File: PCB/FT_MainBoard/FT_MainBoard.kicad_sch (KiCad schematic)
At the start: 7 parts

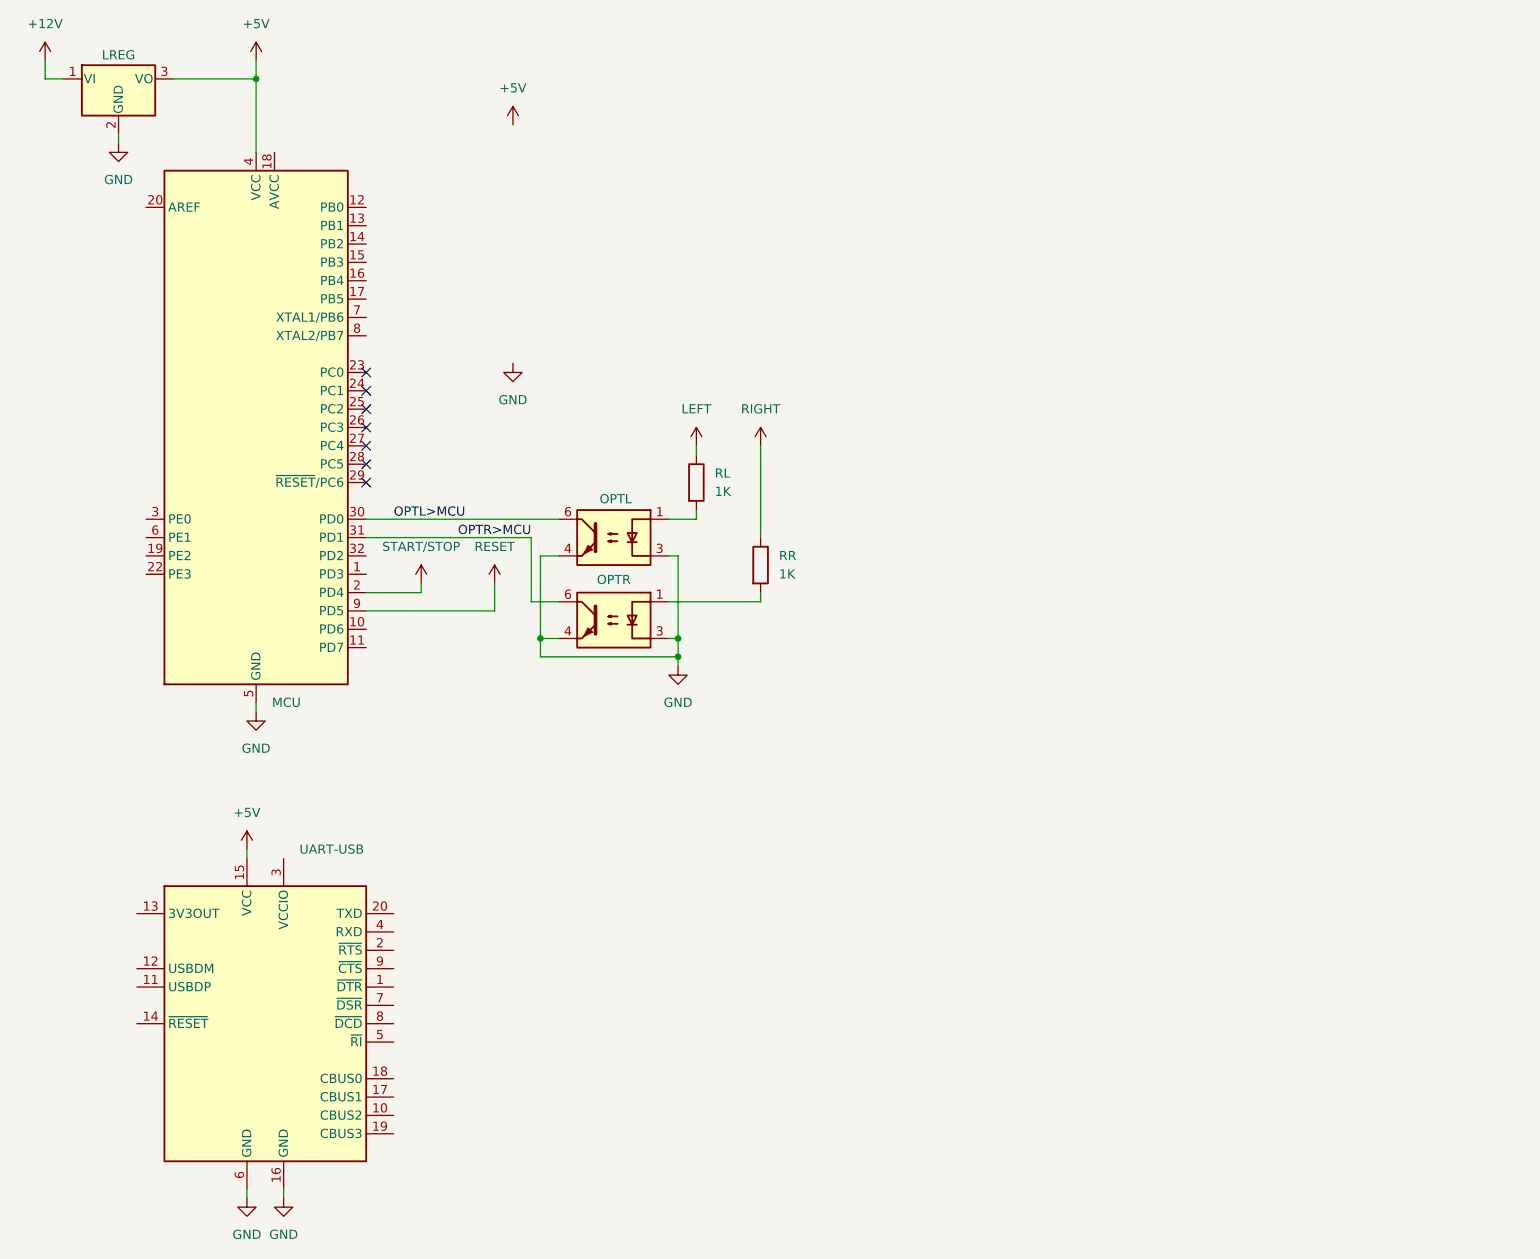
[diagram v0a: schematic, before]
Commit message: update mb shematic
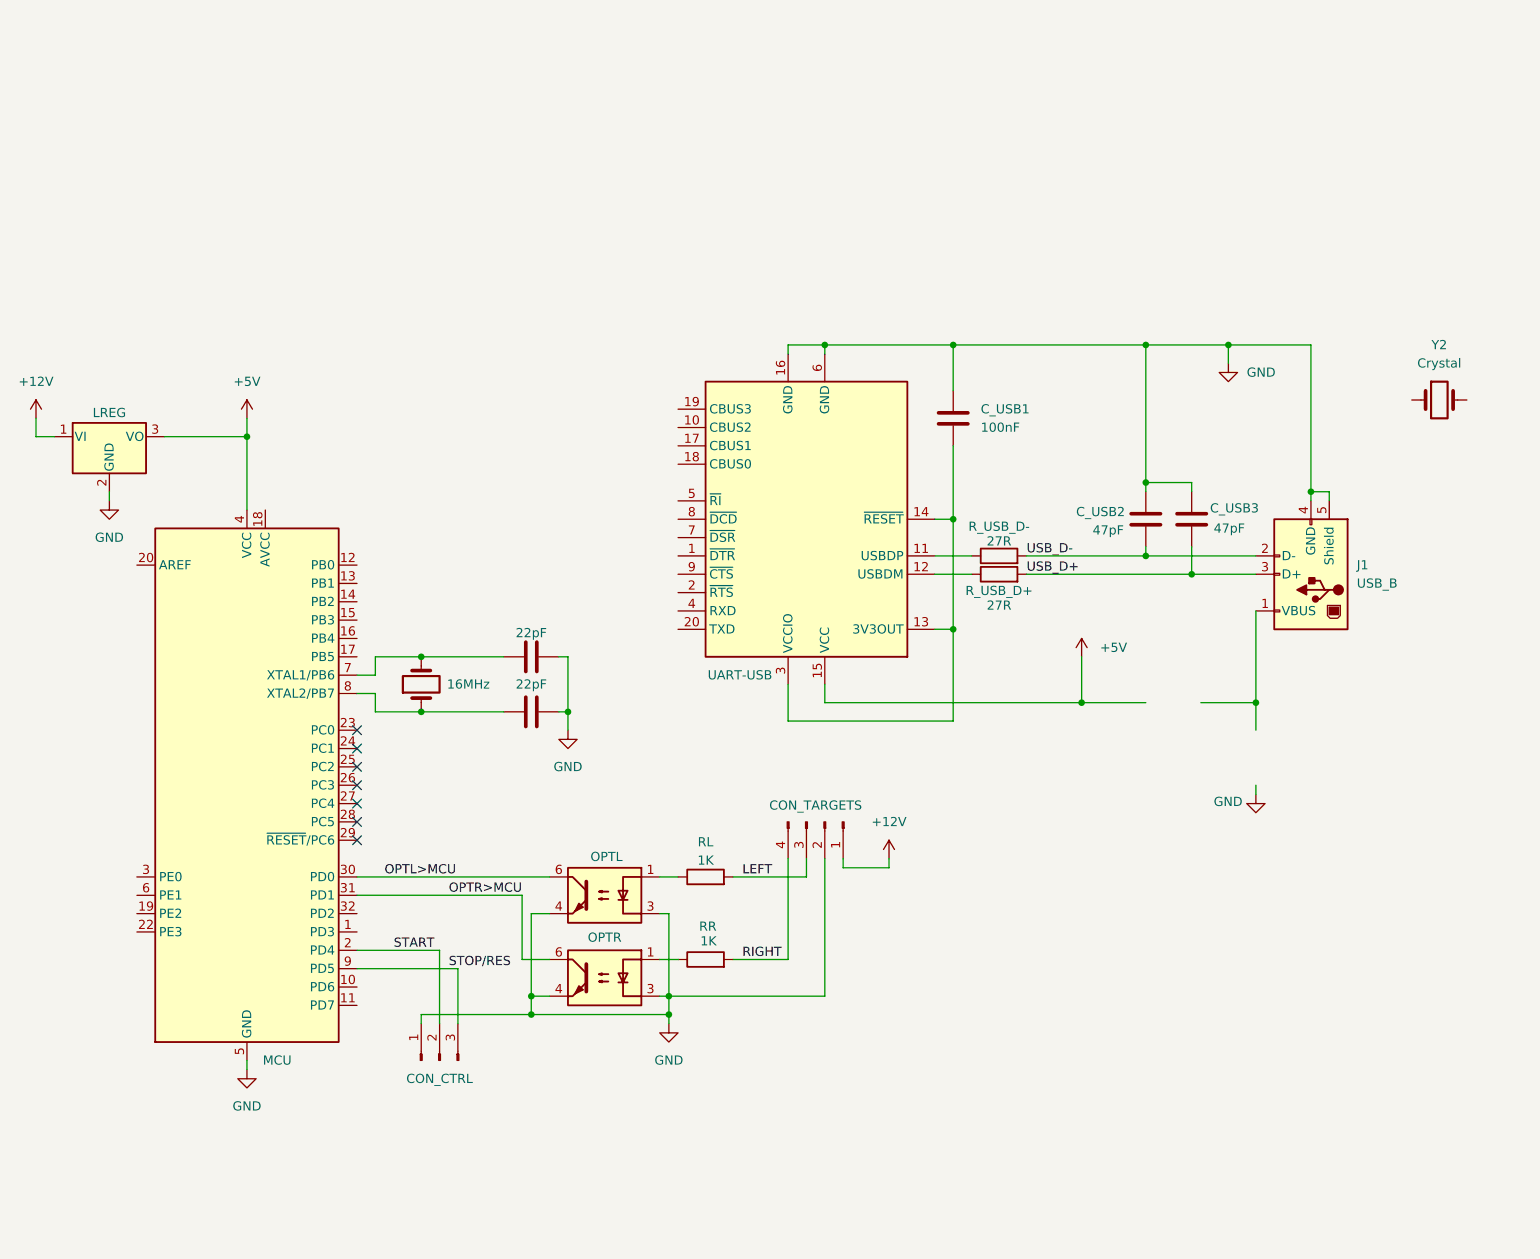
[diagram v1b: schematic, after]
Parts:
- added CON_CTRL: Conn_01x03_Pin, Connector:FanPinHeader_1x03_P2.54mm_Vertical, symbol Connector:Conn_01x03_Pin
- added CON_TARGETS: Conn_01x04_Pin, Connector:FanPinHeader_1x04_P2.54mm_Vertical, symbol Connector:Conn_01x04_Pin
- added C_MCU_OSC1, C_MCU_OSC2: 22pF, symbol Device:C
- added C_USB1: 100nF, symbol Device:C
- added C_USB2, C_USB3: 47pF, symbol Device:C
- added J1: USB_B, symbol Connector:USB_B
- added MCU_OSC: 16MHz, Crystal:Crystal_SMD_HC49-SD_HandSoldering, symbol Device:Crystal
- added R_USB_D+, R_USB_D-: 27R, symbol Device:R
- added Y2: Crystal, Crystal:Crystal_SMD_HC49-SD_HandSoldering, symbol Device:Crystal
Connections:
- net +12V: now also CON_TARGETS.1 (Pin_1)
- net GND: now also CON_CTRL.1 (Pin_1), CON_TARGETS.2 (Pin_2), C_MCU_OSC1.2, C_MCU_OSC2.2, C_USB1.1, C_USB2.1, C_USB3.1, J1.4 (GND), J1.5 (Shield)
- net LEFT: now also RL.2, CON_TARGETS.3 (Pin_3); no longer RL.1
- net RIGHT: now also RR.2, CON_TARGETS.4 (Pin_4); no longer RR.1
- net at OPTL.1: now also RL.1; no longer RL.2
- net at OPTR.1: now also RR.1; no longer RR.2
- net at MCU.7 (XTAL1/PB6): now also C_MCU_OSC1.1, MCU_OSC.2
- net at MCU.8 (XTAL2/PB7): now also C_MCU_OSC2.1, MCU_OSC.1
- net at UART-USB.11 (USBDP): now also R_USB_D-.1
- net at UART-USB.12 (USBDM): now also R_USB_D+.1
- net at UART-USB.13 (3V3OUT): now also UART-USB.14 (~{RESET}), UART-USB.3 (VCCIO), C_USB1.2
- net RESET renamed STOP/RES
- net STOP/RES: now also CON_CTRL.3 (Pin_3)
- net START/STOP renamed START
- net START: now also CON_CTRL.2 (Pin_2)
- new net USB_D+: C_USB3.2, J1.3 (D+), R_USB_D+.2
- new net USB_D-: C_USB2.2, J1.2 (D-), R_USB_D-.2
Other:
- moved on the sheet: LREG, MCU, OPTL, OPTR, RL, RR, UART-USB

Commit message: main board corruption fix
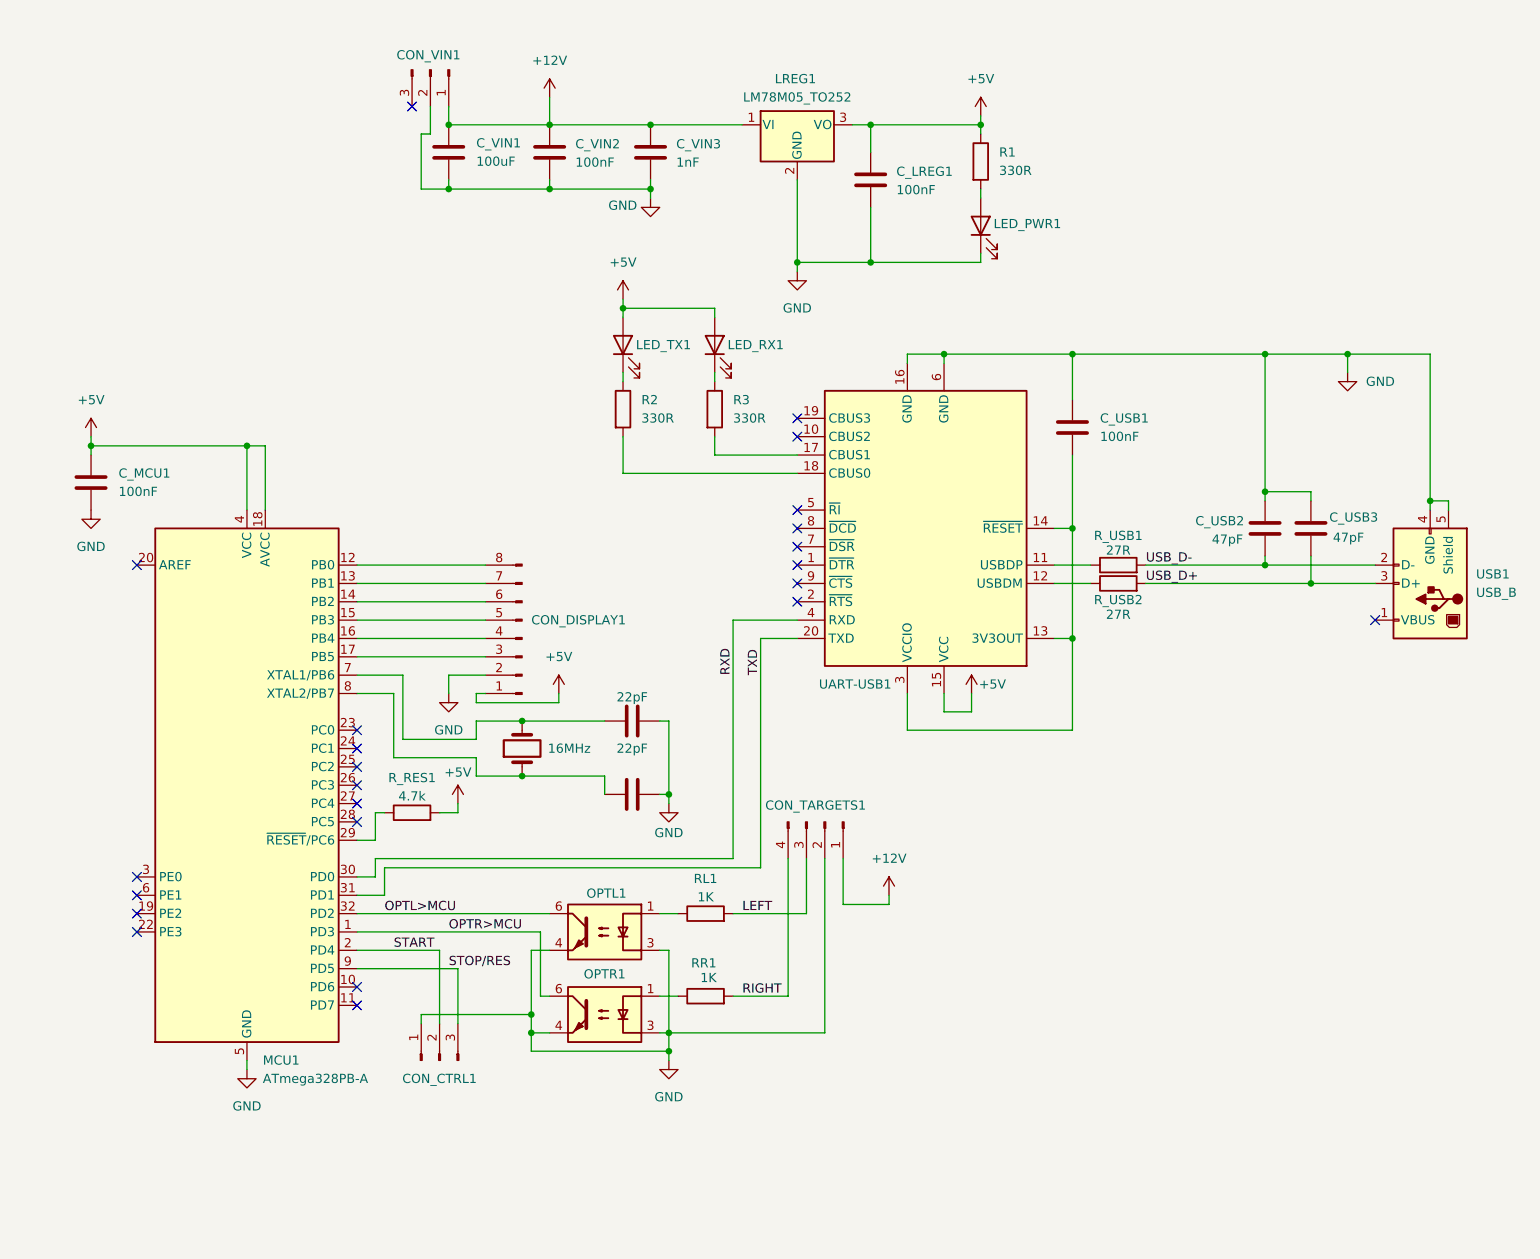
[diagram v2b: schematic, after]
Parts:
- removed Y2: Crystal, Crystal:Crystal_SMD_HC49-SD_HandSoldering, symbol Device:Crystal
- added CON_DISPLAY1: Conn_01x08_Pin, Connector_PinSocket_2.54mm:PinSocket_1x08_P2.54mm_Vertical, symbol Connector:Conn_01x08_Pin
- added CON_VIN1: Conn_01x03_Pin, Connector:FanPinHeader_1x03_P2.54mm_Vertical, symbol Connector:Conn_01x03_Pin
- added C_LREG1, C_MCU1, C_VIN2: 100nF, Capacitor_SMD:C_0603_1608Metric_Pad1.08x0.95mm_HandSolder, symbol Device:C
- added C_VIN1: 100uF, Capacitor_SMD:C_1206_3216Metric_Pad1.33x1.80mm_HandSolder, symbol Device:C
- added C_VIN3: 1nF, Capacitor_SMD:C_0603_1608Metric_Pad1.08x0.95mm_HandSolder, symbol Device:C
- added LED_PWR1: RED, LED_SMD:LED_0603_1608Metric_Pad1.05x0.95mm_HandSolder, symbol Device:LED
- added LED_RX1: YELLOW, LED_SMD:LED_0603_1608Metric_Pad1.05x0.95mm_HandSolder, symbol Device:LED
- added LED_TX1: GREEN, LED_SMD:LED_0603_1608Metric_Pad1.05x0.95mm_HandSolder, symbol Device:LED
- added R1, R2, R3: 330R, Resistor_SMD:R_0603_1608Metric_Pad0.98x0.95mm_HandSolder, symbol Device:R
- added R_RES1: 4.7k, Resistor_SMD:R_0603_1608Metric_Pad0.98x0.95mm_HandSolder, symbol Device:R
- C_MCU_OSC1, C_MCU_OSC2, C_USB1, C_USB2, C_USB3: footprint (none) -> Capacitor_SMD:C_0603_1608Metric_Pad1.08x0.95mm_HandSolder
- MCU_OSC1: renamed from MCU_OSC; footprint Crystal:Crystal_SMD_HC49-SD_HandSoldering -> Crystal:Crystal_SMD_3225-4Pin_3.2x2.5mm_HandSoldering
- R_USB1: renamed from R_USB_D-; footprint (none) -> Resistor_SMD:R_0603_1608Metric_Pad0.98x0.95mm_HandSolder
- R_USB2: renamed from R_USB_D+; footprint (none) -> Resistor_SMD:R_0603_1608Metric_Pad0.98x0.95mm_HandSolder
- USB1: renamed from J1; footprint (none) -> Connector_USB:USB_B_Lumberg_2411_02_Horizontal
- renumbered CON_CTRL to CON_CTRL1, CON_TARGETS to CON_TARGETS1, LREG to LREG1, MCU to MCU1, OPTL to OPTL1, OPTR to OPTR1, RL to RL1, RR to RR1, UART-USB to UART-USB1
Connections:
- net +12V: now also CON_VIN1.1 (Pin_1), C_VIN1.1, C_VIN2.1, C_VIN3.1
- net +5V: now also MCU1.18 (AVCC), CON_DISPLAY1.1 (Pin_1), C_LREG1.1, C_MCU1.1, LED_RX1.2 (A), LED_TX1.2 (A), R1.1, R_RES1.2
- net GND: now also CON_DISPLAY1.2 (Pin_2), CON_VIN1.2 (Pin_2), C_LREG1.2, C_MCU1.2, C_VIN1.2, C_VIN2.2, C_VIN3.2, LED_PWR1.1 (K)
- net OPTL>MCU: now also MCU1.32 (PD2); no longer MCU1.30 (PD0)
- net OPTR>MCU: now also MCU1.1 (PD3); no longer MCU1.31 (PD1)
- net at MCU1.12 (PB0): now also CON_DISPLAY1.8 (Pin_8)
- net at MCU1.13 (PB1): now also CON_DISPLAY1.7 (Pin_7)
- net at MCU1.14 (PB2): now also CON_DISPLAY1.6 (Pin_6)
- net at MCU1.15 (PB3): now also CON_DISPLAY1.5 (Pin_5)
- net at MCU1.16 (PB4): now also CON_DISPLAY1.4 (Pin_4)
- net at MCU1.17 (PB5): now also CON_DISPLAY1.3 (Pin_3)
- net at MCU1.29 (~{RESET}/PC6): now also R_RES1.1
- net at UART-USB1.17 (CBUS1): now also R3.2
- net at UART-USB1.18 (CBUS0): now also R2.2
- net TXD: now reaches UART-USB1.20 (TXD)
- net TXD: now also MCU1.31 (PD1)
- net RXD: now reaches UART-USB1.4 (RXD)
- net RXD: now also MCU1.30 (PD0)
- new net: LED_PWR1.2 (A), R1.2
- new net: LED_TX1.1 (K), R2.1
- new net: LED_RX1.1 (K), R3.1
- no-connect marks 7 -> 23
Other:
- moved on the sheet: C_USB1, C_USB2, C_USB3, LREG1, OPTL1, OPTR1, RL1, RR1, R_USB1, R_USB2, UART-USB1, USB1
